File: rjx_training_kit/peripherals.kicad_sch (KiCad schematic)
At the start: 18 parts, among them Q7 BC847, SW3 SW_Push, U2 BME280, U3 DS3231M, U5 LIS3DH

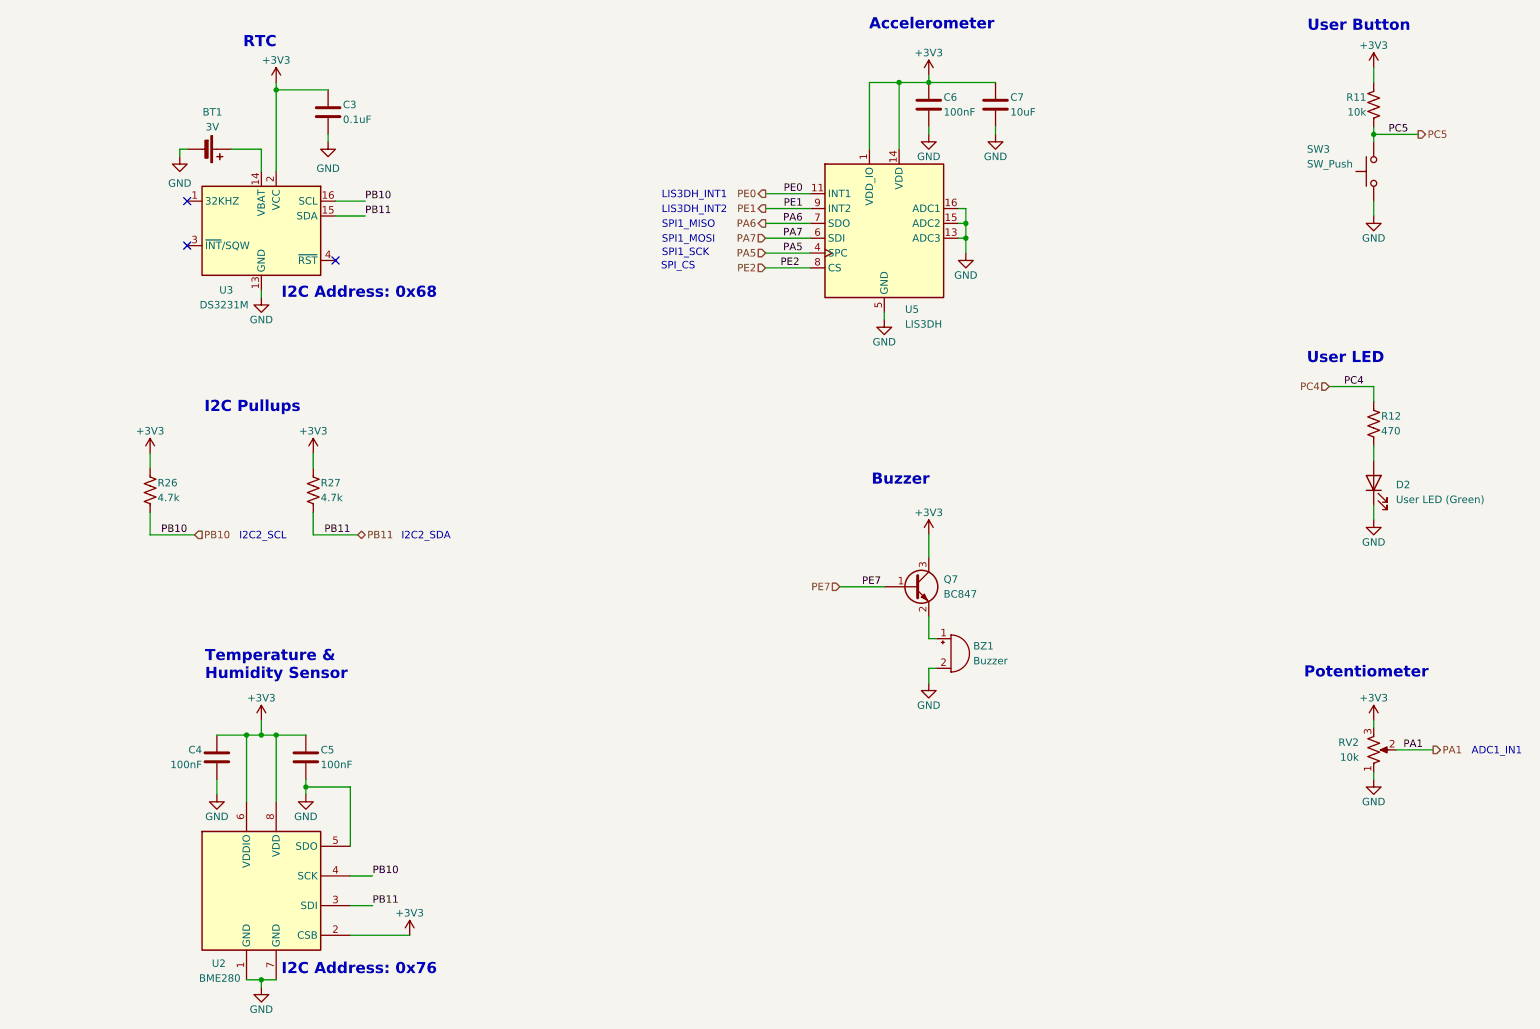
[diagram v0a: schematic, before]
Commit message: Update
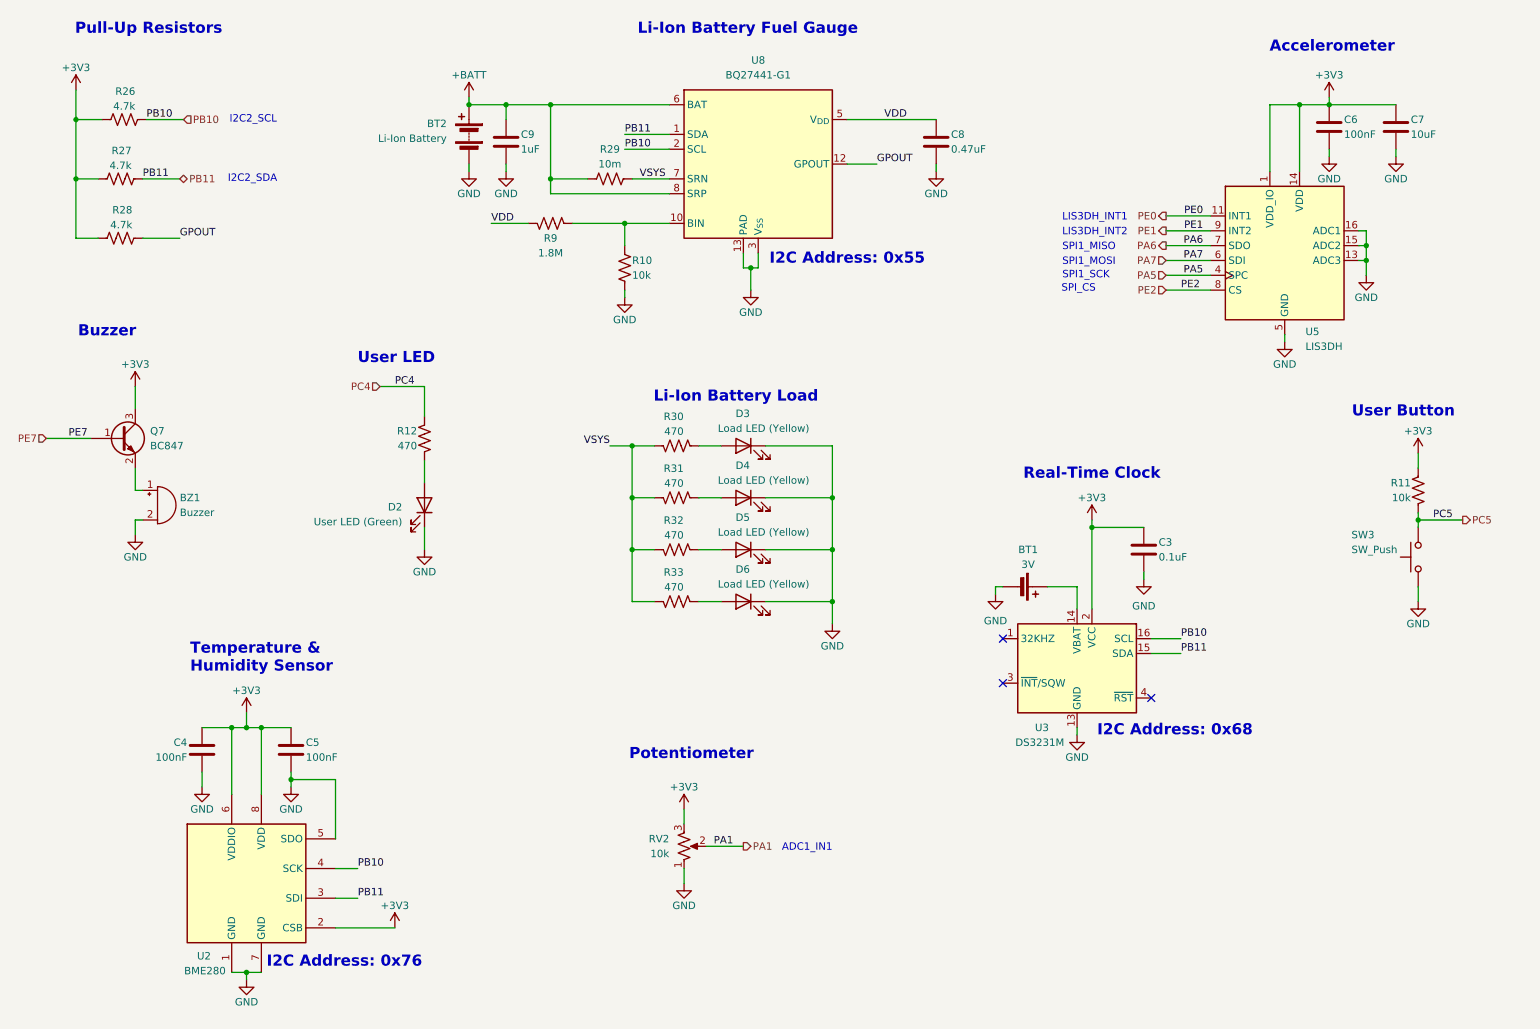
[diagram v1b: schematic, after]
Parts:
- added BT2: Li-Ion Battery, symbol Device:Battery
- added C8: 0.47uF, symbol Device:C
- added C9: 1uF, symbol Device:C
- added D3, D4, D5, D6: Load LED (Yellow), symbol Device:LED
- added R10: 10k, symbol Device:R_US
- added R28: 4.7k, symbol Device:R_US
- added R29: 10m, symbol Device:R_US
- added R30, R31, R32, R33: 470, symbol Device:R_US
- added R9: 1.8M, symbol Device:R_US
- added U8: BQ27441-G1, Package_SON:Texas_S-PDSO-N12, symbol Battery_Management:BQ27441-G1
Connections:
- net +3V3: now also R28.1
- net GND: now also BT2.2 (-), C8.2, C9.2, D3.1 (K), D4.1 (K), D5.1 (K), D6.1 (K), R10.2, U8.13 (PAD), U8.3 (V_{SS})
- net PB10: now also U8.2 (SCL)
- net PB11: now also U8.1 (SDA)
- new net: D3.2 (A), R30.2
- new net: D4.2 (A), R31.2
- new net: D5.2 (A), R32.2
- new net: R10.1, R9.2, U8.10 (BIN)
- new net: D6.2 (A), R33.2
- new net +BATT: BT2.1 (+), C9.1, R29.1, U8.6 (BAT), U8.8 (SRP)
- new net GPOUT: R28.2, U8.12 (GPOUT)
- new net VDD: C8.1, R9.1, U8.5 (V_{DD})
- new net VSYS: R29.2, R30.1, R31.1, R32.1, R33.1, U8.7 (SRN)
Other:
- note added: "I2C Address: 0x55"
- note added: "Li-Ion Battery Fuel Gauge"
- note added: "Li-Ion Battery Load"
- note added: "Pull-Up Resistors"
- note added: "Real-Time Clock"
- note removed: "I2C Pullups"
- note removed: "RTC"
- moved on the sheet: BT1, BZ1, C3, C4, C5, C6, C7, D2, Q7, R11, R12, R26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
